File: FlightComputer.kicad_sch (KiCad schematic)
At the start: 4 parts

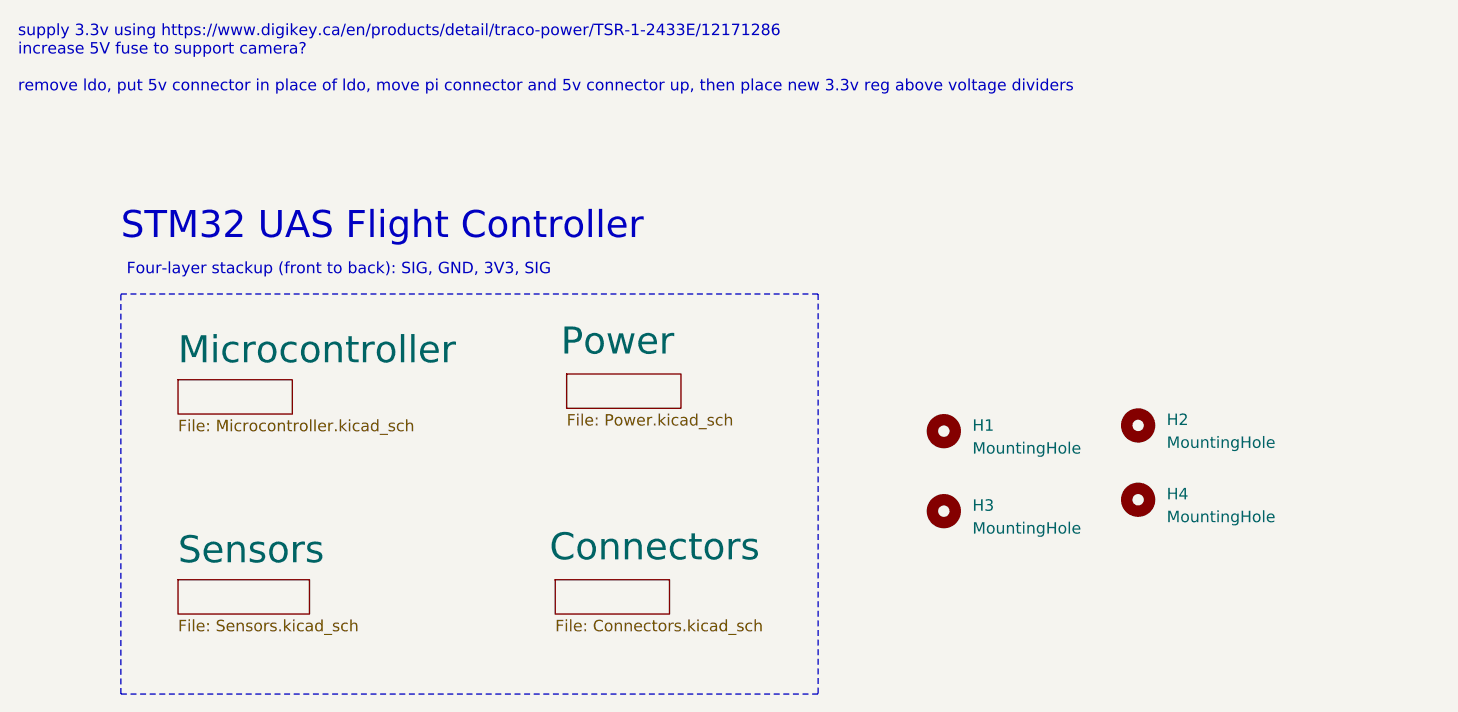
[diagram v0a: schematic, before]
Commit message: Add files via upload
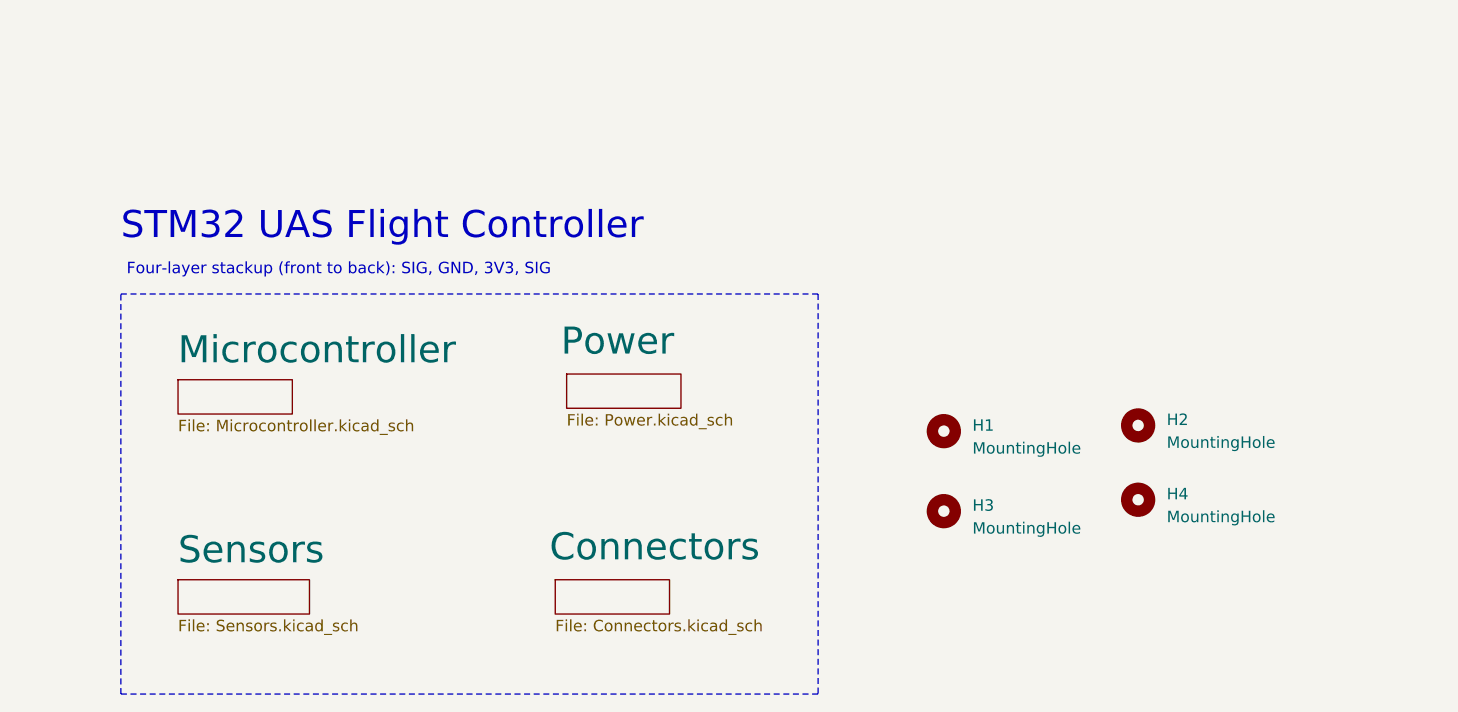
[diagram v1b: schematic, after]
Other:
- note removed: "supply 3.3v using https://www.digikey.ca/en/products/detail/traco-power/TSR-1-2433E/12171286 increase 5V fuse to support camera? remove ldo, put 5v connector in place of ldo, move pi connector and 5v connector up, then place new 3.3v reg above voltage dividers"
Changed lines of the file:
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@@
     (fill (type none))
-  )
-  (text "supply 3.3v using https://www.digikey.ca/en/products/detail/traco-power/TSR-1-2433E/12171286\nincrease 5V fuse to support camera?\n\nremove ldo, put 5v connector in place of ldo, move pi connector and 5v connector up, then place new 3.3v reg above voltage dividers"
-    (at 26.035 24.765 0)
-    (effects (font (size 1.27 1.27)) (justify left bottom))
   )
   (text "Four-layer stackup (front to back): SIG, GND, 3V3, SIG"

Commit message: Add files via upload
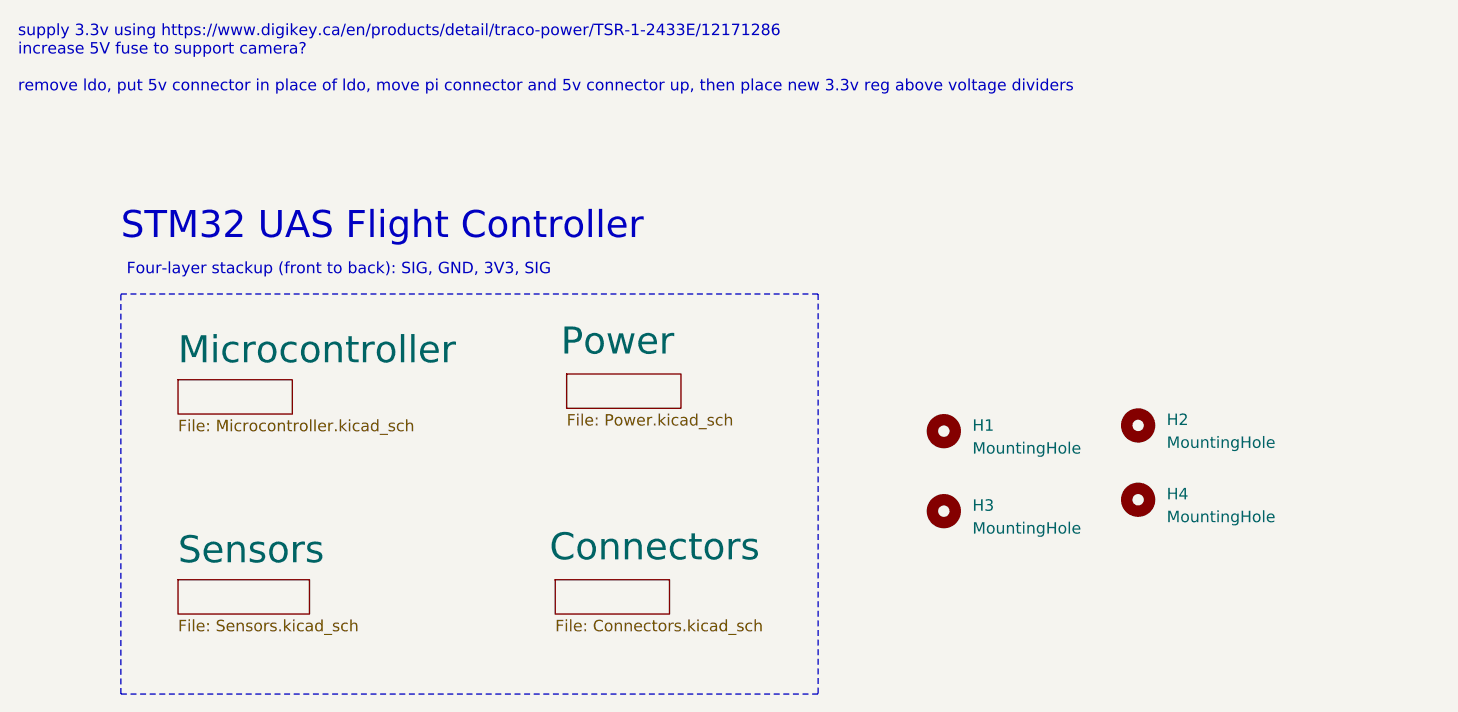
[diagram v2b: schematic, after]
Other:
- note added: "supply 3.3v using https://www.digikey.ca/en/products/detail/traco-power/TSR-1-2433E/12171286 increase 5V fuse to support camera? remove ldo, put 5v connector in place of ldo, move pi connector and 5v connector up, then place new 3.3v reg above voltage dividers"
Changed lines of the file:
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@@
     (fill (type none))
+  )
+  (text "supply 3.3v using https://www.digikey.ca/en/products/detail/traco-power/TSR-1-2433E/12171286\nincrease 5V fuse to support camera?\n\nremove ldo, put 5v connector in place of ldo, move pi connector and 5v connector up, then place new 3.3v reg above voltage dividers"
+    (at 26.035 24.765 0)
+    (effects (font (size 1.27 1.27)) (justify left bottom))
   )
   (text "Four-layer stackup (front to back): SIG, GND, 3V3, SIG"
